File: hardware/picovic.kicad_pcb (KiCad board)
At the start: 2 copper layers, 54.6 x 53.3 mm, 13 parts, among them J1 Mini-DIN-6, J2 DB15_Female_HighDensity, U1 Pico, U2 SN74LVC4245A

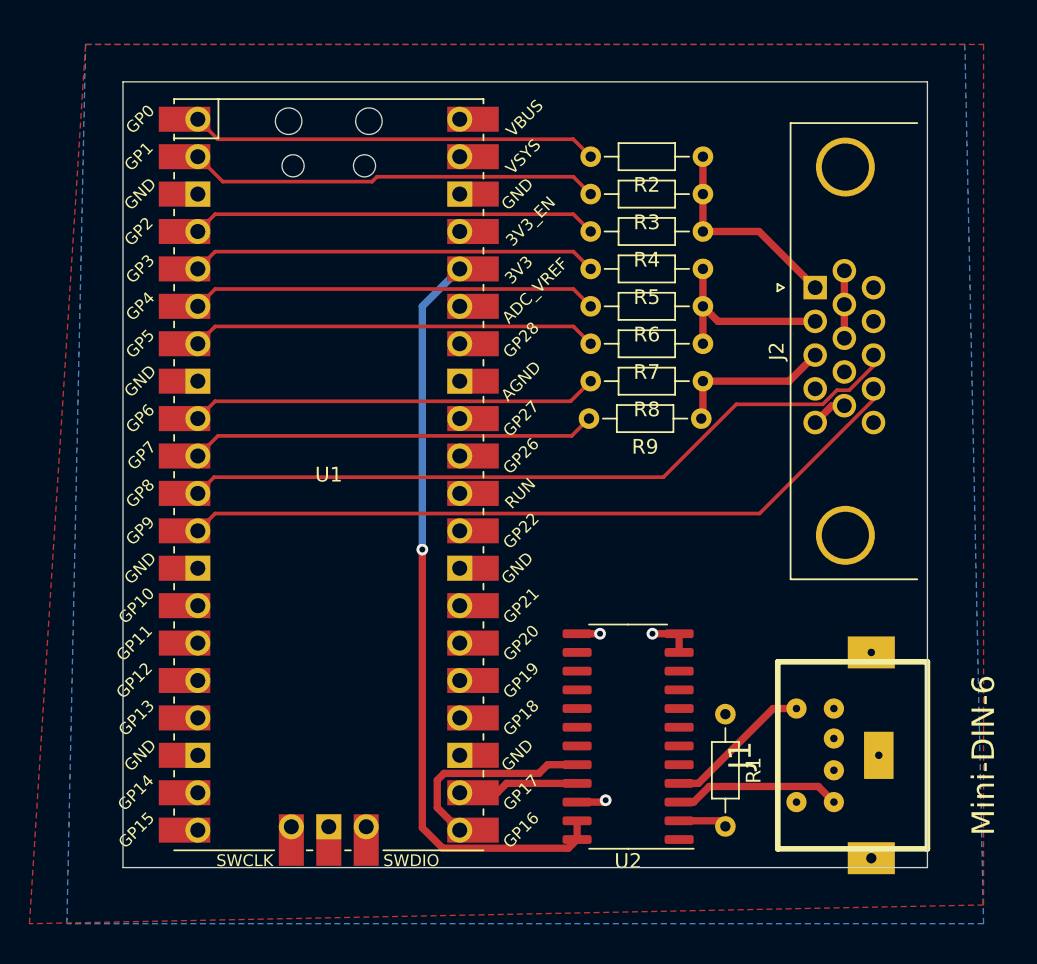
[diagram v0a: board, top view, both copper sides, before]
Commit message: PCB
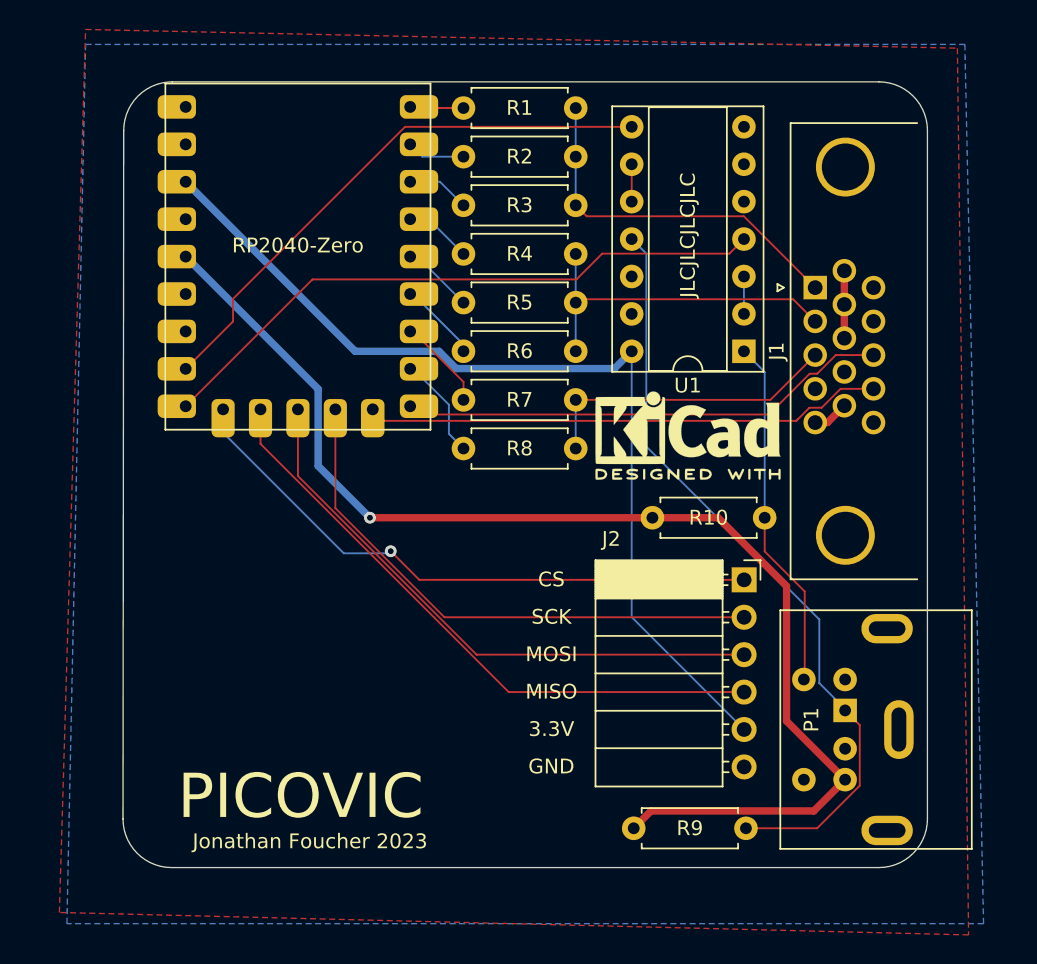
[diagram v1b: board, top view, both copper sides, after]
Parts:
- removed the J1 at (76.2, 36.8)
- removed the R1 at (67.6, 34.0)
- removed U2: SN74LVC4245A, Package_SO:SO-24_5.3x15mm_P1.27mm
- added J2: Conn_01x06, Connector_PinSocket_2.54mm:PinSocket_1x06_P2.54mm_Horizontal, F.Cu at (68.8, 24.9)
- added P1: Mini-DIN_6pins_ver2, Custom_Footprints:Connector_Mini-DIN_Female_6Pin_2rows, F.Cu at (75.7, 33.8)
- added R10: R, Resistor_THT:R_Axial_DIN0207_L6.3mm_D2.5mm_P7.62mm_Horizontal, F.Cu at (62.6, 20.7)
- added R9: R, Resistor_THT:R_Axial_DIN0207_L6.3mm_D2.5mm_P7.62mm_Horizontal, F.Cu at (61.3, 41.8)
- added REF**: KiCad-Logo2_5mm_SilkScreen, Symbol:KiCad-Logo2_5mm_SilkScreen, F.Cu at (65.0, 15.1)
- added RZ1: RP2040-Zero, RP2040-Zero:RP2040-Zero, F.Cu at (28.4, 15.7)
- R1: renamed from R2; value R_Small -> 1k; footprint Resistor_THT:R_Axial_DIN0204_L3.6mm_D1.6mm_P7.62mm_Horizontal -> Resistor_THT:R_Axial_DIN0207_L6.3mm_D2.5mm_P7.62mm_Horizontal
- R2: renamed from R3; value R_Small -> 500R; footprint Resistor_THT:R_Axial_DIN0204_L3.6mm_D1.6mm_P7.62mm_Horizontal -> Resistor_THT:R_Axial_DIN0207_L6.3mm_D2.5mm_P7.62mm_Horizontal
- R3: renamed from R4; value R_Small -> 250R; footprint Resistor_THT:R_Axial_DIN0204_L3.6mm_D1.6mm_P7.62mm_Horizontal -> Resistor_THT:R_Axial_DIN0207_L6.3mm_D2.5mm_P7.62mm_Horizontal
- R4: renamed from R5; value R_Small -> 1k; footprint Resistor_THT:R_Axial_DIN0204_L3.6mm_D1.6mm_P7.62mm_Horizontal -> Resistor_THT:R_Axial_DIN0207_L6.3mm_D2.5mm_P7.62mm_Horizontal
- R5: renamed from R6; value R_Small -> 500R; footprint Resistor_THT:R_Axial_DIN0204_L3.6mm_D1.6mm_P7.62mm_Horizontal -> Resistor_THT:R_Axial_DIN0207_L6.3mm_D2.5mm_P7.62mm_Horizontal
- R6: renamed from R7; value R_Small -> 250R; footprint Resistor_THT:R_Axial_DIN0204_L3.6mm_D1.6mm_P7.62mm_Horizontal -> Resistor_THT:R_Axial_DIN0207_L6.3mm_D2.5mm_P7.62mm_Horizontal
- R7: renamed from R8; value R_Small -> 500R; footprint Resistor_THT:R_Axial_DIN0204_L3.6mm_D1.6mm_P7.62mm_Horizontal -> Resistor_THT:R_Axial_DIN0207_L6.3mm_D2.5mm_P7.62mm_Horizontal
- R8: renamed from R9; value R_Small -> 250R; footprint Resistor_THT:R_Axial_DIN0204_L3.6mm_D1.6mm_P7.62mm_Horizontal -> Resistor_THT:R_Axial_DIN0207_L6.3mm_D2.5mm_P7.62mm_Horizontal
- U1: value Pico -> 74HC14; footprint MCU_RaspberryPi_and_Boards:RPi_Pico_SMD_TH -> Package_DIP:DIP-14_W7.62mm_Socket
- moved U1 29.4 mm to (68.8, 9.40), turned to 180 degrees
- moved R1 9.25 mm to (57.4, -7.11)
- moved R2 9.00 mm to (57.4, -3.81)
- moved R3 8.82 mm to (57.4, -0.51)
- moved R8 8.76 mm to (57.4, 16.0)
- moved R7 8.73 mm to (57.4, 12.7)
- moved R4 8.70 mm to (57.4, 2.79)
- moved R6 8.65 mm to (57.4, 9.40)
- moved R5 8.64 mm to (57.4, 6.10)
- renumbered J2 to J1
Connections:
- J1 pad 11: Net-(J2-Pad11) -> unconnected-(J1-Pad11)
- J1 pad 12: Net-(J2-Pad12) -> unconnected-(J1-Pad12)
- J1 pad 13: Net-(J2-Pad13) -> Net-(J1-Pad13)
- J1 pad 14: Net-(J2-Pad14) -> Net-(J1-Pad14)
- J1 pad 15: Net-(J2-Pad15) -> unconnected-(J1-Pad15)
- J1 pad 4: Net-(J2-Pad4) -> unconnected-(J1-Pad4)
- J1 pad 9: Net-(J2-Pad9) -> unconnected-(J1-Pad9)
- R1 pad 2: Net-(R2-Pad2) -> Net-(R1-Pad2)
- R2 pad 2: Net-(R3-Pad2) -> Net-(R2-Pad2)
- R3 pad 2: Net-(R4-Pad2) -> Net-(R3-Pad2)
- R4 pad 2: Net-(R5-Pad2) -> Net-(R4-Pad2)
- R5 pad 2: Net-(R6-Pad2) -> Net-(R5-Pad2)
- R6 pad 2: Net-(R7-Pad2) -> Net-(R6-Pad2)
- R7 pad 2: Net-(R8-Pad2) -> Net-(R7-Pad2)
- R8 pad 2: Net-(R9-Pad2) -> Net-(R8-Pad2)
- U1 pad 1: Net-(R2-Pad2) -> Net-(P1-Pad5)
- U1 pad 10: Net-(R9-Pad2) -> Net-(U1-Pad10)
- U1 pad 11: Net-(J2-Pad13) -> Net-(P1-Pad1)
- U1 pad 12: Net-(J2-Pad14) -> unconnected-(U1-Pad12)
- U1 pad 13: Net-(U1-Pad13) -> GND
- U1 pad 14: Net-(U1-Pad14) -> +3.3V
- U1 pad 2: Net-(R3-Pad2) -> Net-(U1-Pad2)
- U1 pad 3: Net-(U1-Pad3) -> Net-(U1-Pad2)
- U1 pad 4: Net-(R4-Pad2) -> Net-(RZ1-Pad15)
- U1 pad 5: Net-(R5-Pad2) -> GND
- U1 pad 6: Net-(R6-Pad2) -> unconnected-(U1-Pad6)
- U1 pad 7: Net-(R7-Pad2) -> GND
- U1 pad 9: Net-(R8-Pad2) -> Net-(U1-Pad10)
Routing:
- net +5V: track 0.00 -> 83.6 mm, vias 0 -> 1
- net +3.3V: track 0.00 -> 64.9 mm
- net Net-(P1-Pad1): track 0.00 -> 52.4 mm
- net Net-(U1-Pad36): track 51.6 -> 0.00 mm, vias 1 -> 0
- net Net-(J2-Pad14): track 50.3 -> 0.00 mm
- net Net-(J2-Pad13): track 50.2 -> 0.00 mm
- net Net-(RZ1-Pad15): track 0.00 -> 42.6 mm
- net /MISO: track 0.00 -> 42.5 mm
- net /CS: track 0.00 -> 41.5 mm, vias 0 -> 1
- net /MOSI: track 0.00 -> 40.2 mm
- net Net-(RZ1-Pad16): track 0.00 -> 38.0 mm
- net /SCK: track 0.00 -> 37.9 mm
- net Net-(J1-Pad14): track 0.00 -> 35.3 mm
- net Net-(J1-Pad13): track 0.00 -> 32.6 mm
- net Net-(R9-Pad2): track 27.6 -> 0.00 mm
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- added copper zone on F.Cu, net GND
- removed copper zone on F.Cu, net +5V
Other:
- outline, holes or cut-outs redrawn
- net class Default removed
- board text added: "3.3V"
- board text added: "CS"
- board text added: "GND"
- board text added: "JLCJLCJLCJLC"
- board text added: "Jonathan Foucher 2023"
- board text added: "MISO"
- board text added: "MOSI"
- board text added: "PICOVIC"
- board text added: "SCK"
